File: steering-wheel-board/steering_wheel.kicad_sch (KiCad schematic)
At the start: 12 parts, among them J1 Connector Type TBD, U1 AP63205WU, U2 MIC5504-3.3YM5, U3 ISO1044BD

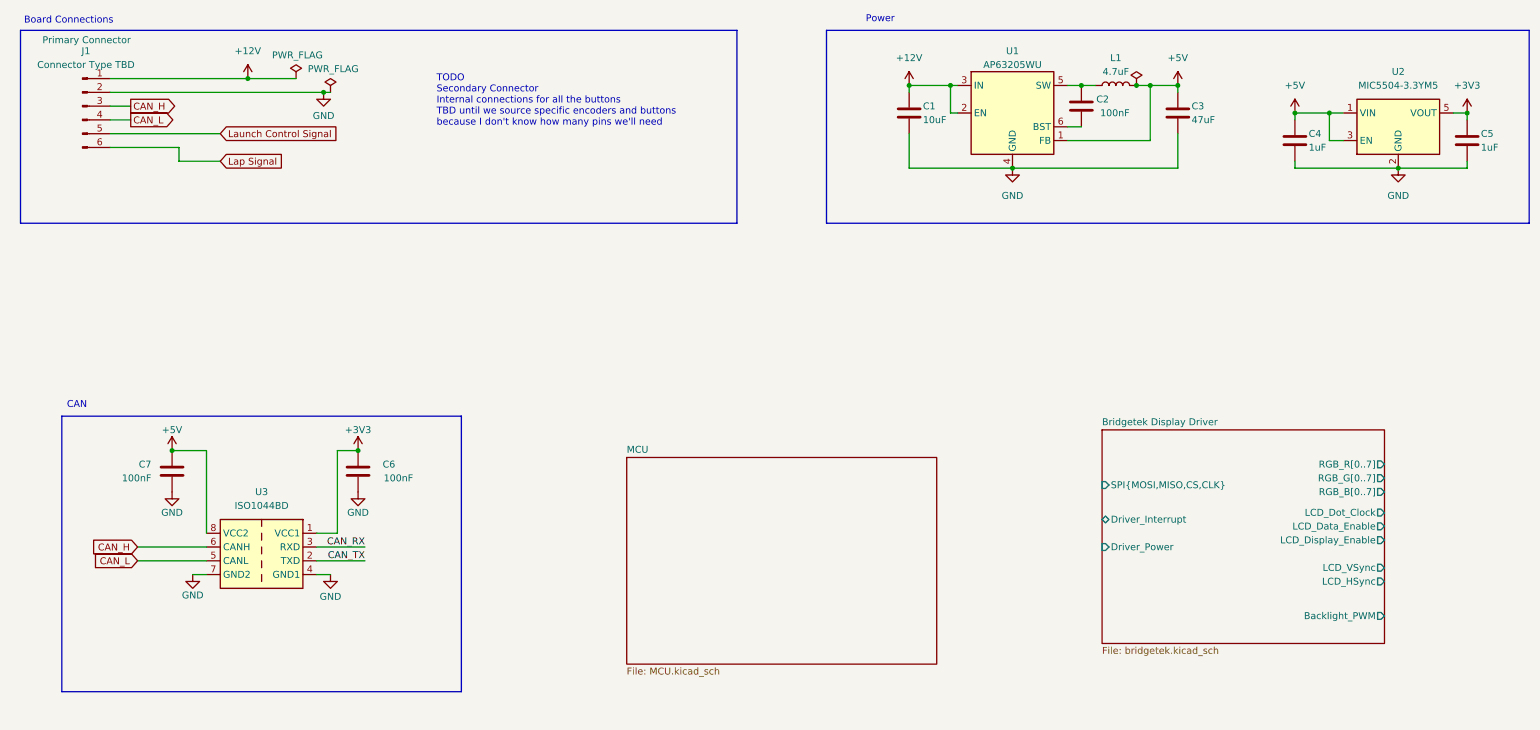
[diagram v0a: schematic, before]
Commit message: MCU page of steering wheel schematic
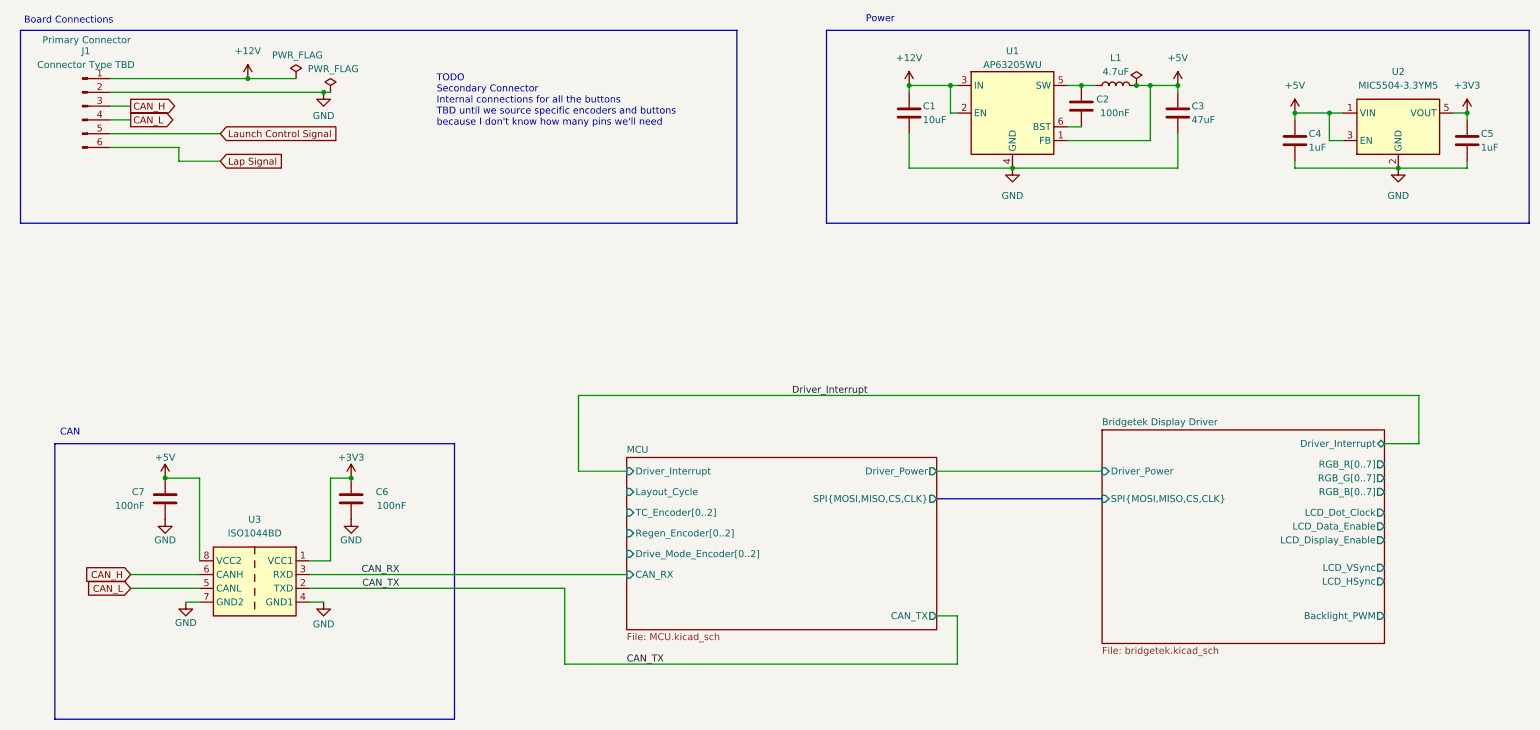
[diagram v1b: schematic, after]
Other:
- sheet MCU ports: added CAN_RX, CAN_TX, Drive_Mode_Encoder[0..2], Driver_Interrupt, Driver_Power, Layout_Cycle, Regen_Encoder[0..2], SPI{MOSI,MISO,CS,CLK}, TC_Encoder[0..2]; removed none
- moved on the sheet: C6, C7, U3
